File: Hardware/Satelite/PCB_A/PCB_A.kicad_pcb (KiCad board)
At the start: 2 copper layers, 47 x 47 mm, 40 parts, among them J1 Batería LiPo (Soldada), J2 CONUFL001-SMD, J3 Servo Globo, J4 Conector_PCB_A-B, J5 Servo Paracaídas, Q1 SSM3J338R,LF, U1 A2235-H, U2 CC1101RGP, U3 0915BM15A0001E, Y1 26 MHz

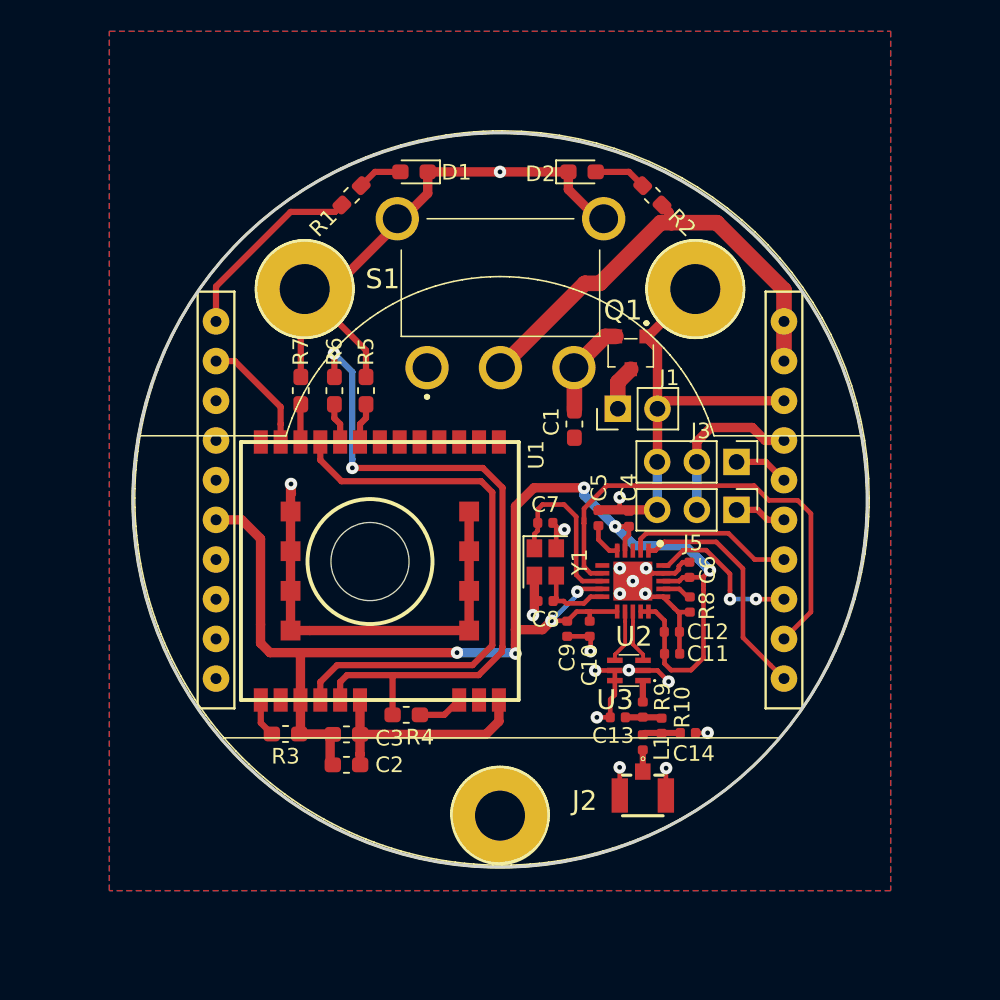
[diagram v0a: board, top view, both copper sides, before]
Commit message: PCB_A terminado
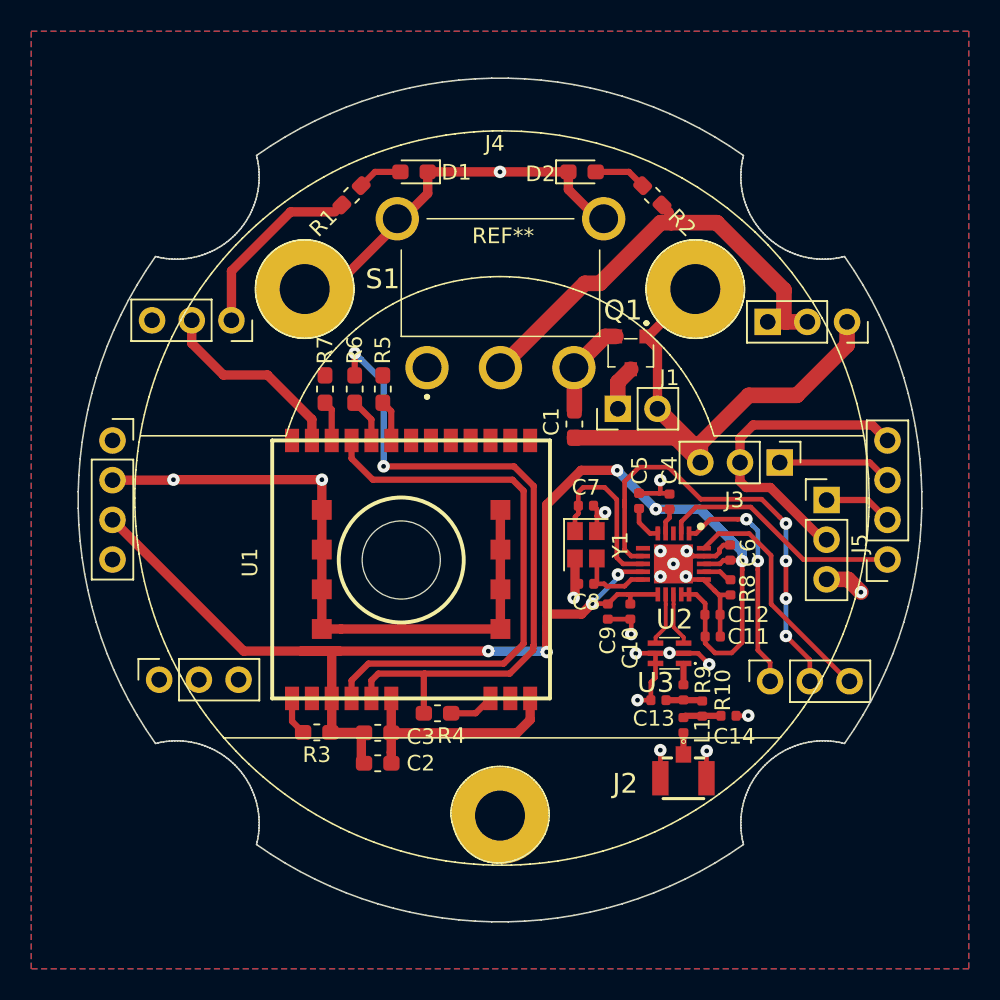
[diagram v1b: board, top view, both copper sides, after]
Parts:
- added REF**: PCB_mayor_diametro, AXTEC:PCB_mayor_diametro, F.Cu at (0.00, 0.00)
- moved J5 5.79 mm to (20.9, 0.00), turned to 0 degrees
- moved C9 2.82 mm to (6.90, 7.14)
- moved C13 2.82 mm to (10.1, 12.8)
- moved C5 2.82 mm to (8.90, 0.06)
- moved C7 2.82 mm to (5.50, 0.36)
- moved J2 2.82 mm to (11.7, 17.8)
- moved C10 2.82 mm to (8.34, 7.14)
- moved C4 2.82 mm to (10.8, 0.10)
- moved R8 2.82 mm to (14.8, 5.59)
- moved U2 2.82 mm to (11.1, 4.09)
- moved Y1 2.82 mm to (5.50, 2.87)
- moved C11 2.82 mm to (13.6, 8.74)
- moved C12 2.82 mm to (13.6, 7.34)
- moved C14 2.82 mm to (14.6, 13.8)
- moved C6 2.82 mm to (14.7, 3.37)
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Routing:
- net GND: track 142.7 -> 154.8 mm, vias 18 -> 20
- net +5V: track 10.7 -> 20.0 mm
- net +3V3_Internal: track 92.4 -> 98.9 mm
- net /SDI: track 10.4 -> 15.6 mm, vias 2 -> 0
- net /SDO: track 10.8 -> 15.7 mm
- net /GPS_TX: track 7.60 -> 12.5 mm
- net /S_GLOBO: track 3.52 -> 7.37 mm
- net /CS: track 30.4 -> 29.0 mm, vias 0 -> 4
- net /S_PARACAIDAS: track 3.30 -> 4.43 mm
- net /SCLK: track 15.1 -> 15.0 mm, vias 0 -> 2
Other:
- board size 47 x 47 mm -> 54 x 54 mm
- net class Alimentacion: trace_width 0.3 -> 0.6
- net class Default: trace_width 0.3 -> 0.4
